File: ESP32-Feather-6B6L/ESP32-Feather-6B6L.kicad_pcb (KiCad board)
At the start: 2 copper layers, 86.4 x 76.2 mm, 36 parts, among them J201 RJ45, J202 RJ45, J401 1 2 3 4 5 6 G, J501 + 1 2 3 4 5 6 -, U201 TCAN332DR, U301 LM2574N-5.0, U403 74HCT14, U501 TBD62084A

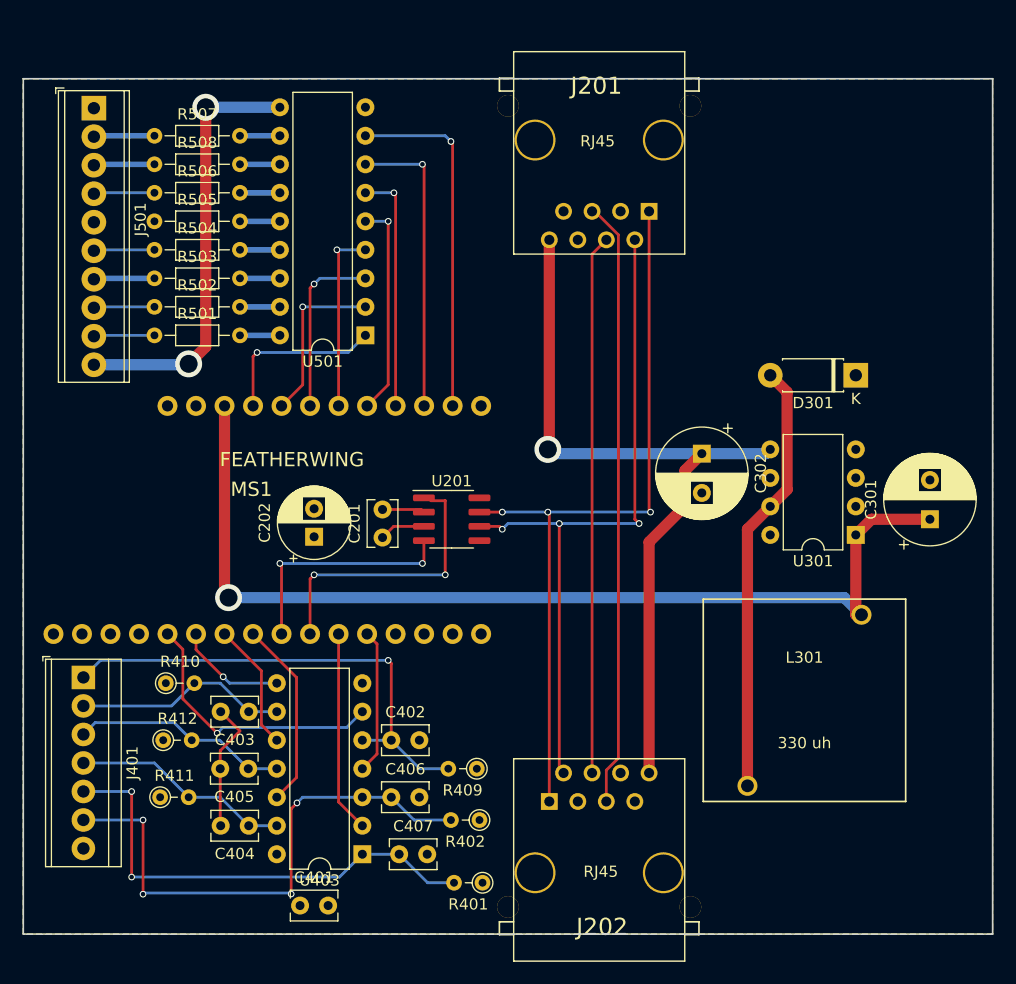
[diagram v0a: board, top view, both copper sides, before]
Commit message: Final through-hole tweaks.
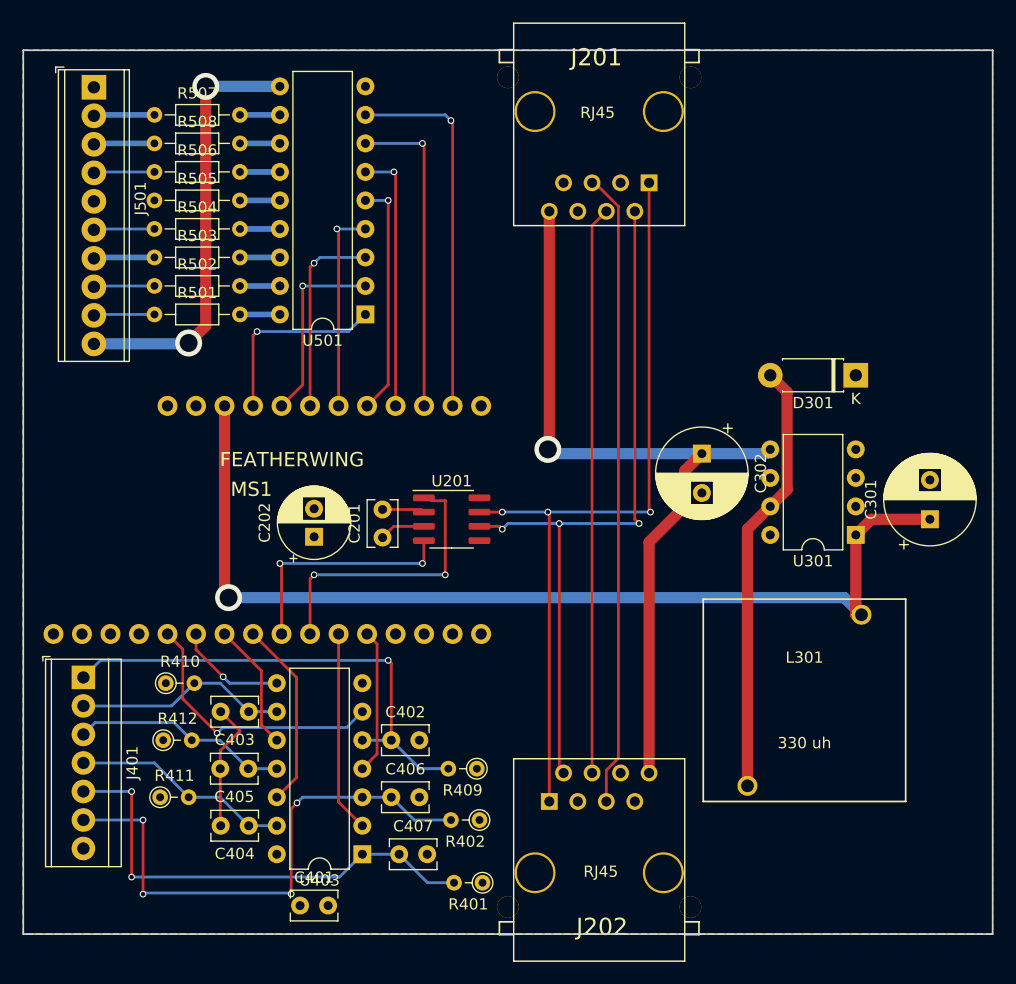
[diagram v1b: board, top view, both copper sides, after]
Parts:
- moved J201 2.54 mm to (178.3, 43.6)
- moved J501 1.86 mm to (133.3, 41.4)
- moved R502 1.86 mm to (138.7, 59.1)
- moved R503 1.86 mm to (138.7, 56.6)
- moved R504 1.86 mm to (138.7, 54.0)
- moved R505 1.86 mm to (138.7, 51.5)
- moved R501 1.86 mm to (138.7, 61.6)
- moved R506 1.86 mm to (138.7, 48.9)
- moved R507 1.86 mm to (138.7, 43.9)
- moved R508 1.86 mm to (138.7, 46.4)
- moved U501 1.86 mm to (157.5, 61.6)
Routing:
- net /CAN Transceiver/CANH: track 67.9 -> 70.5 mm
- net /CAN Transceiver/+12V CAN Power: track 69.2 -> 71.8 mm
- net Net-(J201-Pad5): track 54.1 -> 56.7 mm
- net Net-(J201-Pad4): track 48.0 -> 50.6 mm
- net /CAN Transceiver/CANL: track 62.4 -> 64.9 mm
- net /N$19: track 15.8 -> 17.7 mm
- net /N$3: track 15.2 -> 17.1 mm
- net /N$5: track 15.2 -> 17.1 mm
- net /N$21: track 19.3 -> 21.1 mm
- net /N$24: track 31.4 -> 33.3 mm
- net /N$20: track 16.5 -> 18.4 mm
- net /N$23: track 26.7 -> 28.5 mm
- net /N$22: track 21.6 -> 23.4 mm
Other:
- board size 86.4 x 76.2 mm -> 86.4 x 78.7 mm
